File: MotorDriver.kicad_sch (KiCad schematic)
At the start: 93 parts, among them J1 Screw_Terminal_01x02, J2 Screw_Terminal_01x02, J3 Screw_Terminal_01x02, J4 Conn_01x07_Pin, J5 Conn_01x05_Pin, Q1 PMOS, U1 L298N, U2 INA226, U3 AP63205WU, U4 LM393, U5 AP2112K-3.3, U6 INA226, U7 INA226

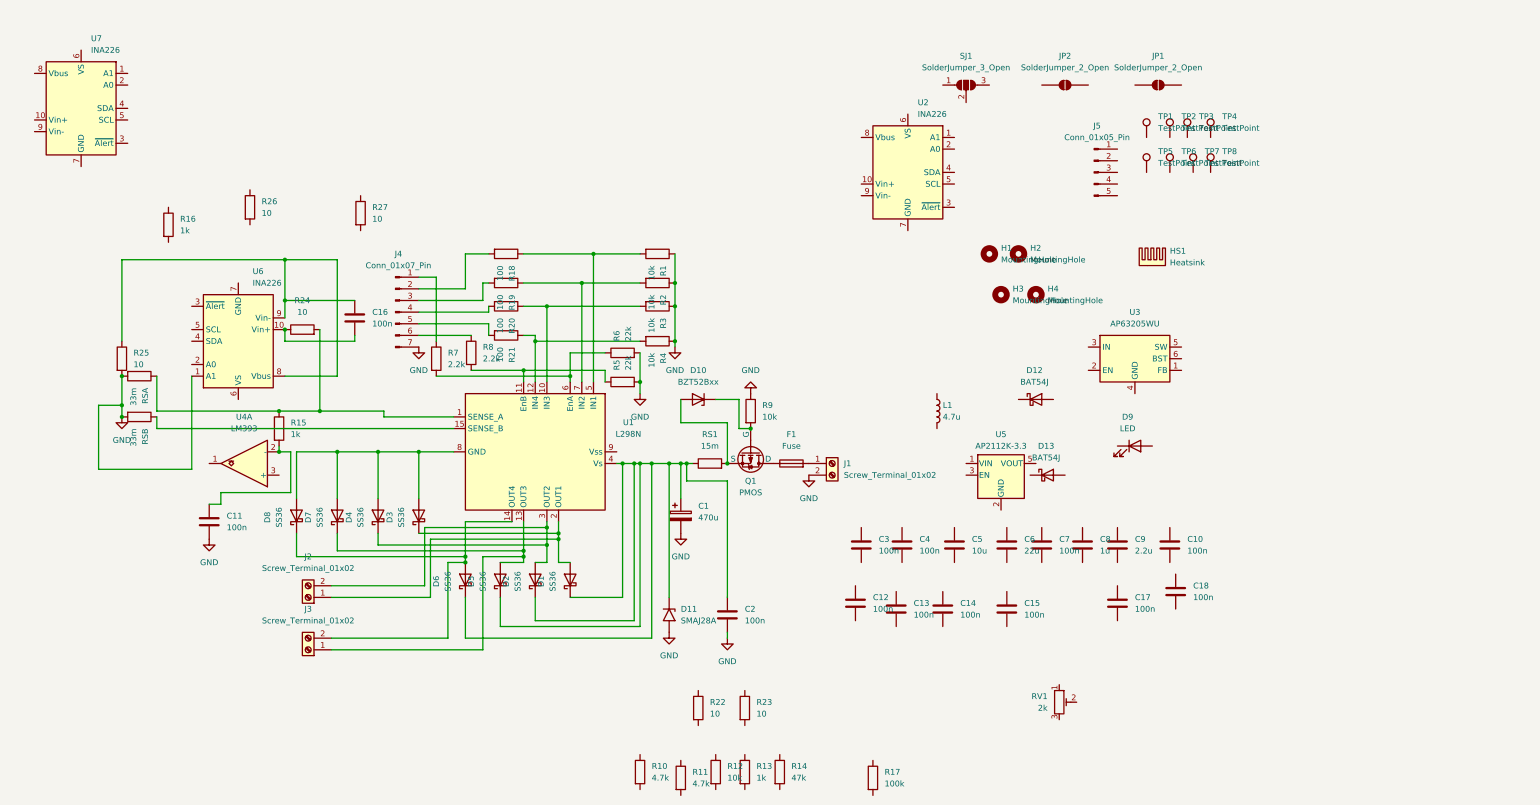
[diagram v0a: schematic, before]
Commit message: final schematic
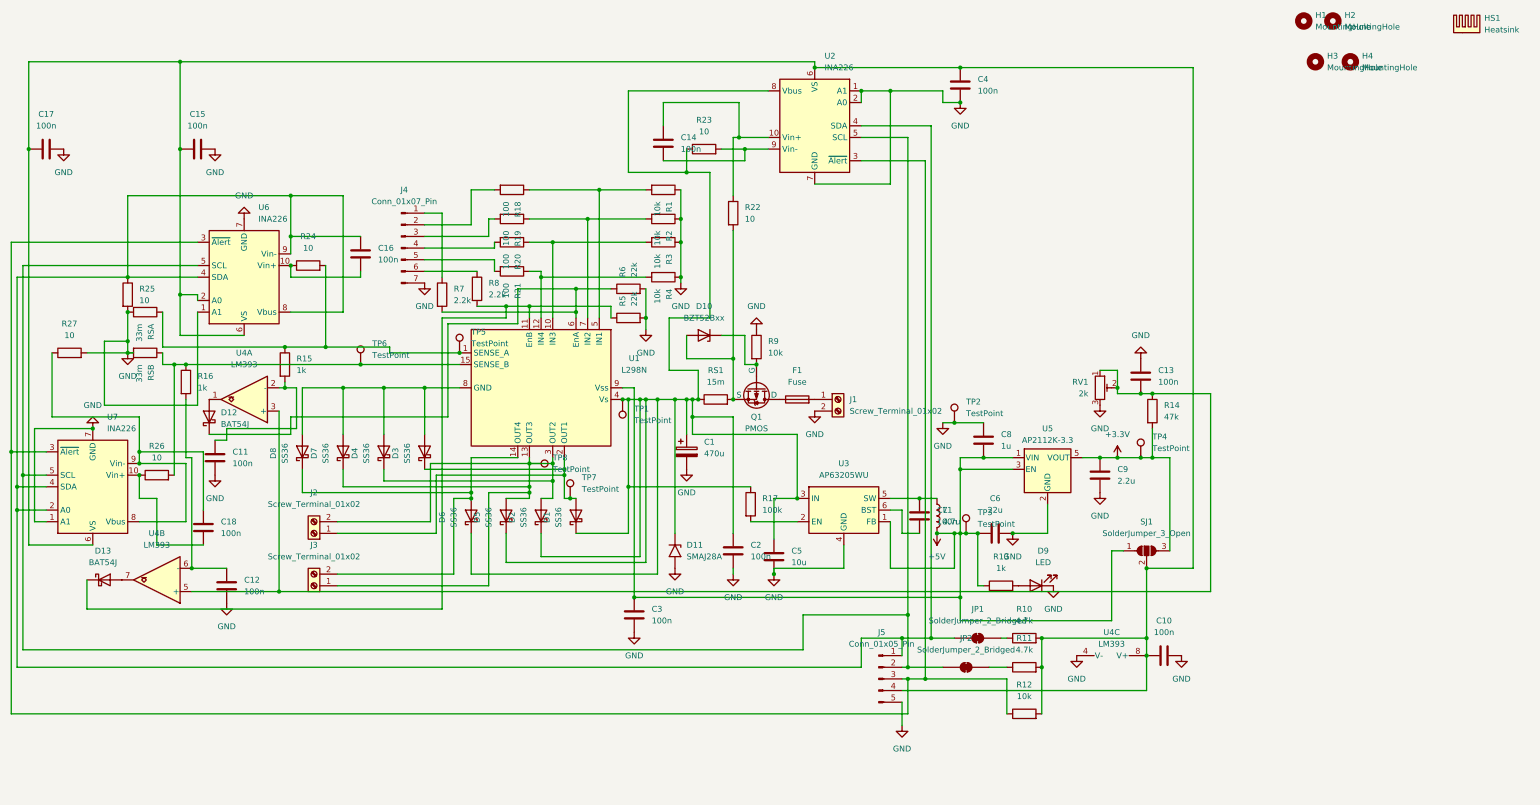
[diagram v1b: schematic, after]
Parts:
- removed JP1, JP2: SolderJumper_2_Open, symbol Jumper:SolderJumper_2_Open
- added JP1, JP2: SolderJumper_2_Bridged, symbol Jumper:SolderJumper_2_Bridged
- added unit 2 of U4
- added unit 3 of U4
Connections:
- net GND: now also C10.2, C12.2, C13.1, C15.2, C17.2, C3.2, C4.2, C5.2, C6.2, C8.1, C9.2, D9.1 (K), J5.5 (Pin_5), R27.2, RV1.3, TP2.1, U2.1 (A1), U2.2 (A0), U2.7 (GND), U3.4 (GND), U5.2 (GND), U6.7 (GND), U7.1 (A1), U7.7 (GND), U4.4 (V-)
- net at C12.1: now also R16.2, U4.6 (-)
- net at C18.1: now also R27.1, U7.8 (Vbus), U7.9 (Vin-)
- net at C18.2: now also R26.1, U7.10 (Vin+)
- net at U2.10 (Vin+): now also C14.1, R22.1
- net at U2.3 (~{Alert}): now also J5.3 (Pin_3), R12.1, U6.3 (~{Alert}), U7.3 (~{Alert})
- net at U2.4 (SDA): now also C16.1, J5.1 (Pin_1), R25.1, U6.4 (SDA), U6.8 (Vbus), U6.9 (Vin-), U7.2 (A0), U7.4 (SDA), JP1.1 (A)
- net at U2.5 (SCL): now also J5.2 (Pin_2), U6.5 (SCL), U7.5 (SCL), JP2.1 (A)
- net at U2.6 (VS): now also C10.1, C15.1, C17.1, C4.1, J5.4 (Pin_4), R10.2, R11.2, R12.2, SJ1.2 (C), U6.2 (A0), U6.6 (VS), U7.6 (VS), U4.8 (V+)
- net at U2.8 (Vbus): now also C1.1, C2.1, C5.1, D1.1 (K), D11.1 (A1), D2.1 (K), D5.1 (K), D6.1 (K), R17.1, R23.1, RS1.1, TP1.1, U1.4 (Vs), U3.3 (IN)
- net at U2.9 (Vin-): now also C14.2, R23.2
- net at D10.2 (A), Q1.3 (S), RS1.2: now also R22.2
- net at R5.1, R8.2, U1.11 (EnB): now also D13.1 (K)
- net at R15.1, R24.2, RSA.1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: now also TP5.1
- net at D5.2 (A), D7.1 (K), J3.1 (Pin_1)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: now also D2.2 (A), D4.1 (K), J2.2 (Pin_2), TP8.1, U1.3 (OUT2)
- net at RSB.1, U1.15 (SENSE_B): now also R16.1, R26.2, TP6.1
- net at D1.2 (A), D3.1 (K), J2.1 (Pin_1)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: now also TP7.1
- net at R6.1, R7.2, U1.6 (EnA): now also D12.1 (K)
- net +5V: now reaches U1.9 (Vss)
- net +5V: now also C3.1, C6.1, C8.2, L1.2, R13.1, SJ1.1 (A), TP3.1, U3.1 (FB), U5.1 (VIN), U5.3 (EN)
- net at D9.2 (A): now also R13.2
- net at R17.2: now also U3.2 (EN)
- net at D12.2 (A): now also U4.1
- net +3.3V: now reaches TP4.1
- net +3.3V: now also C9.1, R14.2, SJ1.3 (B), U5.5 (VOUT)
- net at R11.1: now also JP2.2 (B)
- net at U3.5 (SW): now also C7.1, L1.1
- net at U3.6 (BST): now also C7.2
- net at C13.2: now also R14.1, RV1.1, RV1.2, U4.3 (+), U4.5 (+)
- net at D13.2 (A): now also U4.7
- net at R10.1: now also JP1.2 (B)
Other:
- moved on the sheet: C1, C10, C11, C12, C13, C14, C15, C16, C17, C18, C2, C3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
